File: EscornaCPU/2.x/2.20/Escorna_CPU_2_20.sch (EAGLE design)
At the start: 92 parts, among them IC1 ULN2803, U2 ESP01, U6 ASM1117-3.3, X1 AK550/2, X1.1 AK550/2

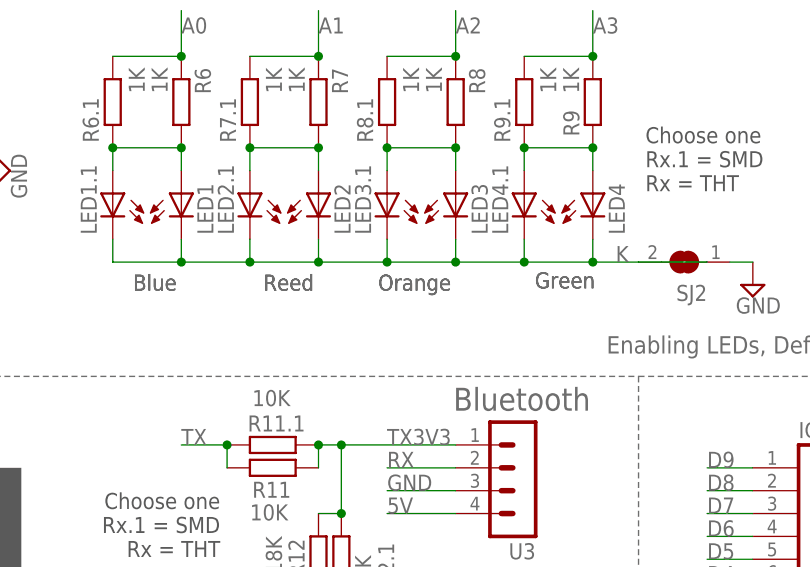
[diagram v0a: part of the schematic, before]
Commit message: Upgrade
cambios en 2.20
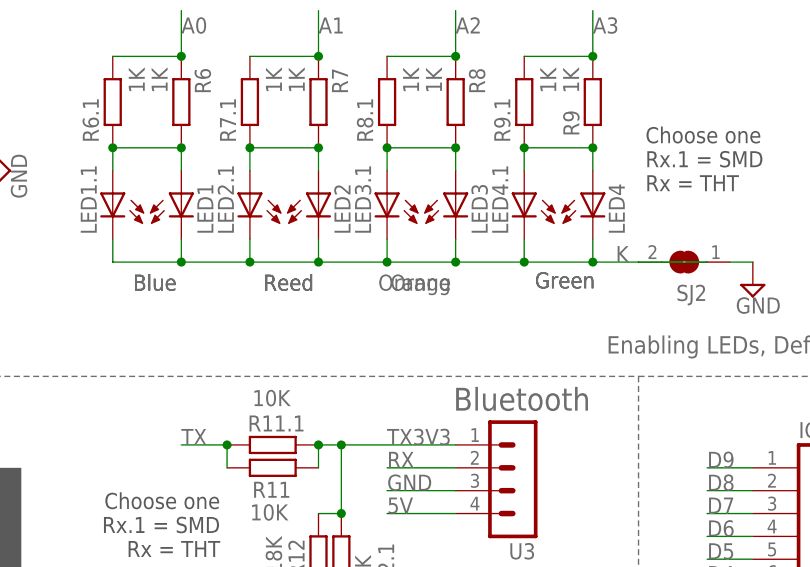
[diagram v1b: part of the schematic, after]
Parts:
- LED3.1: value Orange -> Orang
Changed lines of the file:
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@@
 <part name="LED1.1" library="led" deviceset="LED" device="CHIPLED_0603" value="Blue"/>
 <part name="LED2.1" library="led" deviceset="LED" device="CHIPLED_0603" value="Reed"/>
-<part name="LED3.1" library="led" deviceset="LED" device="CHIPLED_0603" value="Orange"/>
+<part name="LED3.1" library="led" deviceset="LED" device="CHIPLED_0603" value="Orang"/>
 <part name="LED4.1" library="led" deviceset="LED" device="CHIPLED_0603" value="Green"/>
 <part name="JP2" library="SparkFunEagle-6-6-07" deviceset="JP1E" device=""/>
